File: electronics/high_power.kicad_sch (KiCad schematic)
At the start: 40 parts, among them J12 Conn_01x01, J14 Conn_GND, J15 Battery_Conn, J23 Conn_01x01, J24 Conn_01x01, J25 Conn_GND, J29 Conn_GND, J30 Conn_GND, J31 Conn_GND, J4 Conn_01x01, J6 Inverter_Conn, J8 Conn_01x01, U11 INA3221

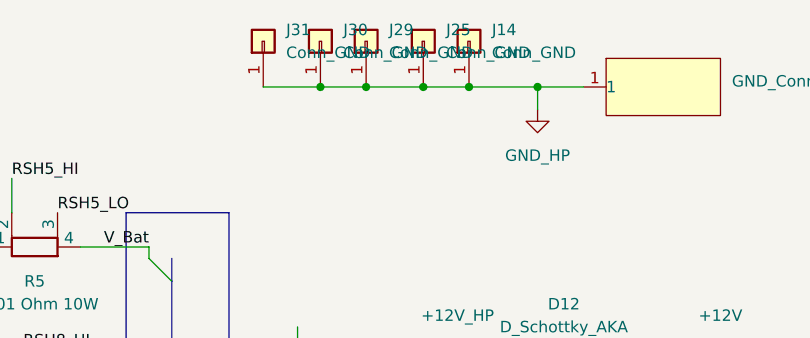
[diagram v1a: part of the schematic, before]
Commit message: layouting progress. some 3d models upload
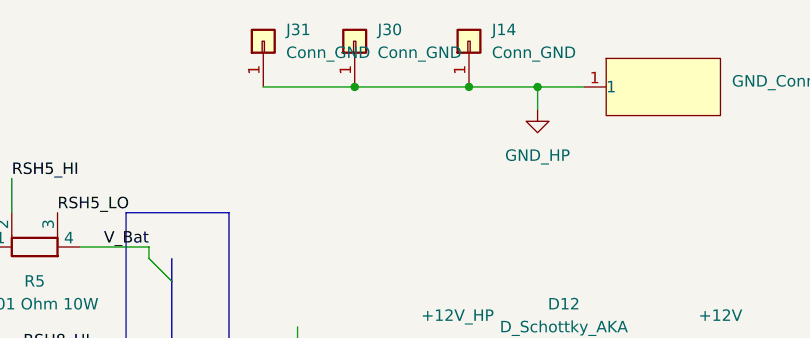
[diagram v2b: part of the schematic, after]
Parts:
- removed J25, J29: Conn_GND, HeavyDuty:keystone_m3_screw_terminal_vertical, symbol Connector_Generic:Conn_01x01
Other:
- moved on the sheet: J30
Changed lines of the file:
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@@
 	)
 	(junction
-		(at 142.24 33.02)
-		(diameter 0)
-		(color 0 0 0 0)
-	)
-	(junction
 		(at 228.6 104.14)
 		(diameter 0)
@@
 	)
 	(junction
-		(at 135.89 33.02)
-		(diameter 0)
-		(color 0 0 0 0)
-	)
-	(junction
 		(at 201.93 135.89)
 		(diameter 0)
@@
 	)
 	(junction
-		(at 130.81 33.02)
-		(diameter 0)
-		(color 0 0 0 0)
-	)
-	(junction
 		(at 116.84 114.3)
 		(diameter 0)
@@
 	)
 	(junction
+		(at 134.62 33.02)
+		(diameter 0)
+		(color 0 0 0 0)
+	)
+	(junction
 		(at 148.59 66.04)
 		(diameter 0)
@@
 	(wire
 		(pts
-			(xy 130.81 33.02) (xy 135.89 33.02)
-		)
-		(stroke
-			(width 0)
-			(type default)
-		)
-	)
-	(wire
-		(pts
 			(xy 148.59 76.2) (xy 148.59 66.04)
 		)
@@
 	(wire
 		(pts
-			(xy 135.89 33.02) (xy 142.24 33.02)
-		)
-		(stroke
-			(width 0)
-			(type default)
-		)
-	)
-	(wire
-		(pts
 			(xy 130.81 177.8) (xy 130.81 180.34)
 		)
@@
 	(wire
 		(pts
+			(xy 134.62 33.02) (xy 147.32 33.02)
+		)
+		(stroke
+			(width 0)
+			(type default)
+		)
+	)
+	(wire
+		(pts
 			(xy 190.5 120.65) (xy 196.85 120.65)
 		)
@@
 	(wire
 		(pts
-			(xy 142.24 33.02) (xy 147.32 33.02)
-		)
-		(stroke
-			(width 0)
-			(type default)
-		)
-	)
-	(wire
-		(pts
 			(xy 256.54 124.46) (xy 252.73 124.46)
 		)
@@
 	(wire
 		(pts
-			(xy 124.46 33.02) (xy 130.81 33.02)
+			(xy 124.46 33.02) (xy 134.62 33.02)
 		)
 		(stroke
@@
 	(label "RSH8_HI"
 		(at 97.79 62.23 0)
+		(fields_autoplaced yes)
 		(effects
 			(font
@@
 	(label "RSH8_LO"
 		(at 176.53 129.54 0)
+		(fields_autoplaced yes)
 		(effects
 			(font
@@
 	(label "RSH8_LO"
 		(at 102.87 64.77 0)
+		(fields_autoplaced yes)
 		(effects
 			(font
@@
 	(label "RSH5_HI"
 		(at 96.52 43.18 0)
+		(fields_autoplaced yes)
 		(effects
 			(font
@@
 	(label "RSH6_HI"
 		(at 176.53 118.11 0)
+		(fields_autoplaced yes)
 		(effects
 			(font
@@
 	(label "V_Bat"
 		(at 116.84 109.22 0)
+		(fields_autoplaced yes)
 		(effects
 			(font
@@
 	(label "V_Bat"
 		(at 111.76 69.85 180)
+		(fields_autoplaced yes)
 		(effects
 			(font
@@
 	(label "VS_INA"
 		(at 266.7 114.3 0)
+		(fields_autoplaced yes)
 		(effects
 			(font
@@
 	(label "RSH5_LO"
 		(at 101.6 46.99 0)
+		(fields_autoplaced yes)
 		(effects
 			(font
@@
 	(label "RSH6_HI"
 		(at 99.06 78.74 0)
+		(fields_autoplaced yes)
 		(effects
 			(font
@@
 	(label "V_Bat"
 		(at 144.78 63.5 180)
+		(fields_autoplaced yes)
 		(effects
 			(font
@@
 	(label "RSH5_HI"
 		(at 176.53 135.89 0)
+		(fields_autoplaced yes)
 		(effects
 			(font
@@
 	(label "RSH6_LO"
 		(at 104.14 81.28 0)
+		(fields_autoplaced yes)
 		(effects
 			(font
@@
 	(label "V_Bat"
 		(at 111.76 50.8 180)
+		(fields_autoplaced yes)
 		(effects
 			(font
@@
 	(label "V_Bat"
 		(at 111.76 85.09 180)
+		(fields_autoplaced yes)
 		(effects
 			(font
@@
 	(label "VS_INA"
 		(at 231.14 104.14 0)
+		(fields_autoplaced yes)
 		(effects
 			(font
@@
 	(label "RSH6_LO"
 		(at 176.53 120.65 0)
+		(fields_autoplaced yes)
 		(effects
 			(font
@@
 	(label "RSH5_LO"
 		(at 176.53 138.43 0)
+		(fields_autoplaced yes)
 		(effects
 			(font
@@
 	(label "RSH8_HI"
 		(at 176.53 127 0)
+		(fields_autoplaced yes)
 		(effects
 			(font
@@
 		(shape bidirectional)
 		(at 273.05 125.73 0)
+		(fields_autoplaced yes)
 		(effects
 			(font
@@
 		(shape bidirectional)
 		(at 273.05 128.27 0)
+		(fields_autoplaced yes)
 		(effects
 			(font
@@
 	(symbol
 		(lib_id "Connector_Generic:Conn_01x01")
-		(at 130.81 27.94 90)
+		(at 134.62 27.94 90)
 		(unit 1)
 		(exclude_from_sim no)
@@
 		(fields_autoplaced yes)
 		(property "Reference" "J30"
-			(at 133.35 26.6699 90)
+			(at 137.16 26.6699 90)
 			(effects
 				(font
@@
 		)
 		(property "Value" "Conn_GND"
-			(at 133.35 29.2099 90)
+			(at 137.16 29.2099 90)
 			(effects
 				(font
@@
 		)
 		(property "Footprint" "HeavyDuty:keystone_m3_screw_terminal_vertical"
-			(at 130.81 27.94 0)
+			(at 134.62 27.94 0)
 			(effects
 				(font
@@
 		)
 		(property "Datasheet" "~"
-			(at 130.81 27.94 0)
+			(at 134.62 27.94 0)
 			(effects
 				(font
@@
 		)
 		(property "Description" "Generic connector, single row, 01x01, script generated (kicad-library-utils/schlib/autogen/connector/)"
-			(at 130.81 27.94 0)
+			(at 134.62 27.94 0)
 			(effects
 				(font
@@
 	)
 	(symbol
-		(lib_id "Connector_Generic:Conn_01x01")
-		(at 135.89 27.94 90)
-		(unit 1)
-		(exclude_from_sim no)
-		(in_bom yes)
-		(on_board yes)
-		(dnp no)
-		(fields_autoplaced yes)
-		(property "Reference" "J29"
-			(at 138.43 26.6699 90)
-			(effects
-				(font
-					(size 1.27 1.27)
-				)
-				(justify right)
-			)
-		)
-		(property "Value" "Conn_GND"
-			(at 138.43 29.2099 90)
-			(effects
-				(font
-					(size 1.27 1.27)
-				)
-				(justify right)
-			)
-		)
-		(property "Footprint" "HeavyDuty:keystone_m3_screw_terminal_vertical"
-			(at 135.89 27.94 0)
-			(effects
-				(font
-					(size 1.27 1.27)
-				)
-				(hide yes)
-			)
-		)
-		(property "Datasheet" "~"
-			(at 135.89 27.94 0)
-			(effects
-				(font
-					(size 1.27 1.27)
-				)
-				(hide yes)
-			)
-		)
-		(property "Description" "Generic connector, single row, 01x01, script generated (kicad-library-utils/schlib/autogen/connector/)"
-			(at 135.89 27.94 0)
-			(effects
-				(font
-					(size 1.27 1.27)
-				)
-				(hide yes)
-			)
-		)
-		(pin "1"
-		)
-		(instances
-			(project "electronics"
-				(path "/eeb1234c-eae0-4ac6-a30d-2a978d66d889/da888cb1-ed89-4b09-bf89-340f462f0940"
-					(reference "J29")
-					(unit 1)
-				)
-			)
-		)
-	)
-	(symbol
 		(lib_id "Device:R_Small")
 		(at 187.96 127 90)
@@
 					(unit 1)
 				)
-			)
-		)
-	)
-	(symbol
-		(lib_id "Connector_Generic:Conn_01x01")
-		(at 142.24 27.94 90)
-		(unit 1)
-		(exclude_from_sim no)
-		(in_bom yes)
-		(on_board yes)
-		(dnp no)
-		(fields_autoplaced yes)
-		(property "Reference" "J25"
-			(at 144.78 26.6699 90)
-			(effects
-				(font
-					(size 1.27 1.27)
-				)
-				(justify right)
-			)
-		)
-		(property "Value" "Conn_GND"
-			(at 144.78 29.2099 90)
-			(effects
-				(font
-					(size 1.27 1.27)
-				)
-				(justify right)
-			)
-		)
-		(property "Footprint" "HeavyDuty:keystone_m3_screw_terminal_vertical"
-			(at 142.24 27.94 0)
-			(effects
-				(font
-					(size 1.27 1.27)
-				)
-				(hide yes)
-			)
-		)
-		(property "Datasheet" "~"
-			(at 142.24 27.94 0)
-			(effects
-				(font
-					(size 1.27 1.27)
-				)
-				(hide yes)
-			)
-		)
-		(property "Description" "Generic connector, single row, 01x01, script generated (kicad-library-utils/schlib/autogen/connector/)"
-			(at 142.24 27.94 0)
-			(effects
-				(font
-					(size 1.27 1.27)
-				)
-				(hide yes)
-			)
-		)
-		(pin "1"
-		)
-		(instances
-			(project "electronics"
-				(path "/eeb1234c-eae0-4ac6-a30d-2a978d66d889/da888cb1-ed89-4b09-bf89-340f462f0940"
-					(reference "J25")
-					(unit 1)
-				)
